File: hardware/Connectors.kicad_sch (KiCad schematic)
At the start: 9 parts, among them J1 USB_C_Receptacle_USB2.0, J14 Conn_01x05, J16 Harw_Conn_2x13, J2 Harw_Conn_1x2, J3 Harw_Conn_1x2, J8 Harw_Conn_1x4

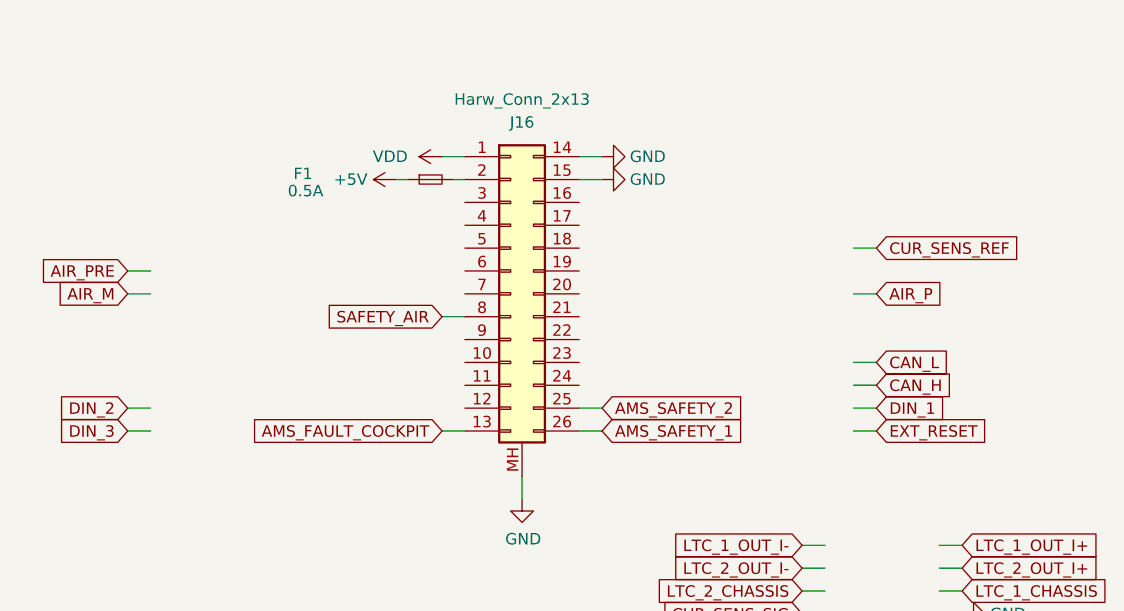
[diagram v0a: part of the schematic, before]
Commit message: pcb update
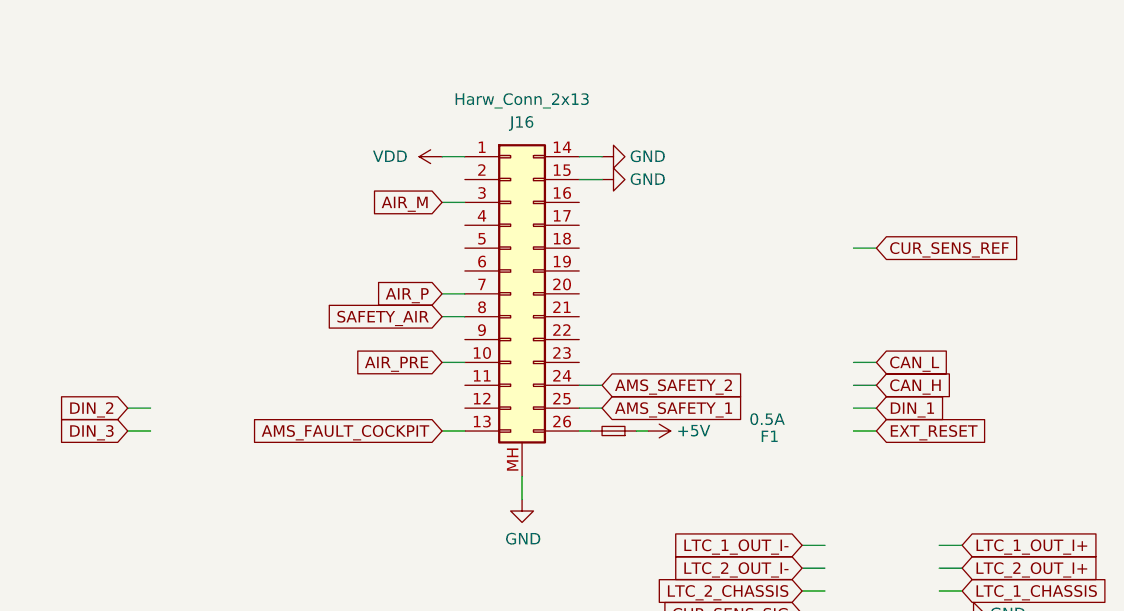
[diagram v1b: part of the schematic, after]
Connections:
- net AIR_M: now also J16.3
- net AIR_P: now also J16.7
- net AIR_PRE: now also J16.10
- net AMS_SAFETY_1: now also J16.25; no longer J16.26
- net AMS_SAFETY_2: now also J16.24; no longer J16.25
- net at F1.2: now also J16.26; no longer J16.2
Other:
- moved on the sheet: F1
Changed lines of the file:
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@@
     (stroke (width 0) (type default) (color 0 0 0 0))
   )
-  (wire (pts (xy 84.455 127) (xy 81.915 127))
+  (wire (pts (xy 84.455 124.46) (xy 81.915 124.46))
     (stroke (width 0) (type default) (color 0 0 0 0))
   )
@@
     (stroke (width 1) (type default) (color 132 0 0 1))
   )
-  (wire (pts (xy 62.865 99.06) (xy 61.595 99.06))
+  (wire (pts (xy 88.265 127) (xy 89.535 127))
     (stroke (width 0) (type default) (color 0 0 0 0))
   )
@@
     (stroke (width 0) (type default) (color 0 0 0 0))
   )
-  (wire (pts (xy 34.29 111.76) (xy 31.75 111.76))
+  (wire (pts (xy 69.215 101.6) (xy 66.675 101.6))
     (stroke (width 0) (type default) (color 0 0 0 0))
   )
@@
     (stroke (width 0) (type default) (color 0 0 0 0))
   )
-  (wire (pts (xy 34.29 109.22) (xy 31.75 109.22))
+  (wire (pts (xy 69.215 119.38) (xy 66.675 119.38))
     (stroke (width 0) (type default) (color 0 0 0 0))
   )
@@
     (stroke (width 0) (type default) (color 0 0 0 0))
   )
-  (wire (pts (xy 69.215 99.06) (xy 67.945 99.06))
+  (wire (pts (xy 81.915 127) (xy 83.185 127))
     (stroke (width 0) (type default) (color 0 0 0 0))
   )
@@
     (stroke (width 0) (type default) (color 0 0 0 0))
   )
-  (wire (pts (xy 112.395 111.76) (xy 114.935 111.76))
+  (wire (pts (xy 69.215 111.76) (xy 66.675 111.76))
     (stroke (width 0) (type default) (color 0 0 0 0))
   )
@@
     (stroke (width 0) (type default) (color 0 0 0 0))
   )
-  (wire (pts (xy 81.915 124.46) (xy 84.455 124.46))
+  (wire (pts (xy 81.915 121.92) (xy 84.455 121.92))
     (stroke (width 0) (type default) (color 0 0 0 0))
   )
@@
     )
   )
-  (global_label "AIR_PRE" (shape input) (at 31.75 109.22 180) (fields_autoplaced)
-    (effects (font (size 1.27 1.27)) (justify right))
-    (property "Intersheet References" "${INTERSHEET_REFS}" (id 0) (at 21.8058 109.2994 0)
+  (global_label "AIR_PRE" (shape input) (at 66.675 119.38 180) (fields_autoplaced)
+    (effects (font (size 1.27 1.27)) (justify right))
+    (property "Intersheet References" "${INTERSHEET_REFS}" (id 0) (at 56.7308 119.4594 0)
       (effects (font (size 1.27 1.27)) (justify right) hide)
     )
@@
     )
   )
-  (global_label "AMS_SAFETY_2" (shape input) (at 84.455 124.46 0) (fields_autoplaced)
+  (global_label "AMS_SAFETY_2" (shape input) (at 84.455 121.92 0) (fields_autoplaced)
+    (effects (font (size 1.27 1.27)) (justify left))
+    (property "Intersheet References" "${INTERSHEET_REFS}" (id 0) (at 100.2654 121.9994 0)
+      (effects (font (size 1.27 1.27)) (justify left) hide)
+    )
+  )
+  (global_label "SWDIO" (shape input) (at 178.435 142.24 180) (fields_autoplaced)
+    (effects (font (size 1.27 1.27)) (justify right))
+    (property "Intersheet References" "${INTERSHEET_REFS}" (id 0) (at 170.2446 142.1606 0)
+      (effects (font (size 1.27 1.27)) (justify right) hide)
+    )
+  )
+  (global_label "AIR_M" (shape input) (at 66.675 101.6 180) (fields_autoplaced)
+    (effects (font (size 1.27 1.27)) (justify right))
+    (property "Intersheet References" "${INTERSHEET_REFS}" (id 0) (at 58.9684 101.6794 0)
+      (effects (font (size 1.27 1.27)) (justify right) hide)
+    )
+  )
+  (global_label "AMS_SAFETY_1" (shape input) (at 84.455 124.46 0) (fields_autoplaced)
     (effects (font (size 1.27 1.27)) (justify left))
     (property "Intersheet References" "${INTERSHEET_REFS}" (id 0) (at 100.2654 124.5394 0)
@@
     )
   )
-  (global_label "SWDIO" (shape input) (at 178.435 142.24 180) (fields_autoplaced)
-    (effects (font (size 1.27 1.27)) (justify right))
-    (property "Intersheet References" "${INTERSHEET_REFS}" (id 0) (at 170.2446 142.1606 0)
-      (effects (font (size 1.27 1.27)) (justify right) hide)
-    )
-  )
-  (global_label "AIR_M" (shape input) (at 31.75 111.76 180) (fields_autoplaced)
-    (effects (font (size 1.27 1.27)) (justify right))
-    (property "Intersheet References" "${INTERSHEET_REFS}" (id 0) (at 24.0434 111.8394 0)
-      (effects (font (size 1.27 1.27)) (justify right) hide)
-    )
-  )
-  (global_label "AMS_SAFETY_1" (shape input) (at 84.455 127 0) (fields_autoplaced)
-    (effects (font (size 1.27 1.27)) (justify left))
-    (property "Intersheet References" "${INTERSHEET_REFS}" (id 0) (at 100.2654 127.0794 0)
-      (effects (font (size 1.27 1.27)) (justify left) hide)
-    )
-  )
   (global_label "D+" (shape input) (at 253.365 114.3 0) (fields_autoplaced)
     (effects (font (size 1.27 1.27)) (justify left))
@@
     )
   )
-  (global_label "AIR_P" (shape input) (at 114.935 111.76 0) (fields_autoplaced)
-    (effects (font (size 1.27 1.27)) (justify left))
-    (property "Intersheet References" "${INTERSHEET_REFS}" (id 0) (at 122.4602 111.6806 0)
-      (effects (font (size 1.27 1.27)) (justify left) hide)
+  (global_label "AIR_P" (shape input) (at 66.675 111.76 180) (fields_autoplaced)
+    (effects (font (size 1.27 1.27)) (justify right))
+    (property "Intersheet References" "${INTERSHEET_REFS}" (id 0) (at 59.1498 111.8394 0)
+      (effects (font (size 1.27 1.27)) (justify right) hide)
     )
   )
@@
     )
   )
-  (symbol (lib_id "Device:Fuse_Small") (at 65.405 99.06 0) (unit 1)
-    (in_bom yes) (on_board yes)
-    (property "Reference" "F1" (id 0) (at 50.165 98.425 0)
+  (symbol (lib_id "Device:Fuse_Small") (at 85.725 127 180) (unit 1)
+    (in_bom yes) (on_board yes)
+    (property "Reference" "F1" (id 0) (at 104.14 127.635 0)
       (effects (font (size 1.27 1.27)) (justify left))
     )
-    (property "Value" "0.5A" (id 1) (at 49.53 100.33 0)
+    (property "Value" "0.5A" (id 1) (at 104.775 125.73 0)
       (effects (font (size 1.27 1.27)) (justify left))
     )
-    (property "Footprint" "Fuse:Fuse_1206_3216Metric" (id 2) (at 65.405 99.06 0)
-      (effects (font (size 1.27 1.27)) hide)
-    )
-    (property "Datasheet" "~" (id 3) (at 65.405 99.06 0)
+    (property "Footprint" "Fuse:Fuse_1206_3216Metric" (id 2) (at 85.725 127 0)
+      (effects (font (size 1.27 1.27)) hide)
+    )
+    (property "Datasheet" "~" (id 3) (at 85.725 127 0)
       (effects (font (size 1.27 1.27)) hide)
     )
@@
     (pin "1")
   )
-  (symbol (lib_id "power:+5V") (at 61.595 99.06 90) (unit 1)
-    (in_bom yes) (on_board yes)
-    (property "Reference" "#PWR03" (id 0) (at 65.405 99.06 0)
-      (effects (font (size 1.27 1.27)) hide)
-    )
-    (property "Value" "+5V" (id 1) (at 56.515 99.06 90))
-    (property "Footprint" "" (id 2) (at 61.595 99.06 0)
-      (effects (font (size 1.27 1.27)) hide)
-    )
-    (property "Datasheet" "" (id 3) (at 61.595 99.06 0)
-      (effects (font (size 1.27 1.27)) hide)
-    )
+  (symbol (lib_id "power:+5V") (at 89.535 127 270) (unit 1)
+    (in_bom yes) (on_board yes)
+    (property "Reference" "#PWR03" (id 0) (at 85.725 127 0)
+      (effects (font (size 1.27 1.27)) hide)
+    )
+    (property "Value" "+5V" (id 1) (at 94.615 127 90))
+    (property "Footprint" "" (id 2) (at 89.535 127 0)
+      (effects (font (size 1.27 1.27)) hide)
+    )
+    (property "Datasheet" "" (id 3) (at 89.535 127 0)
+      (effects (font (size 1.27 1.27)) hide)
+    )

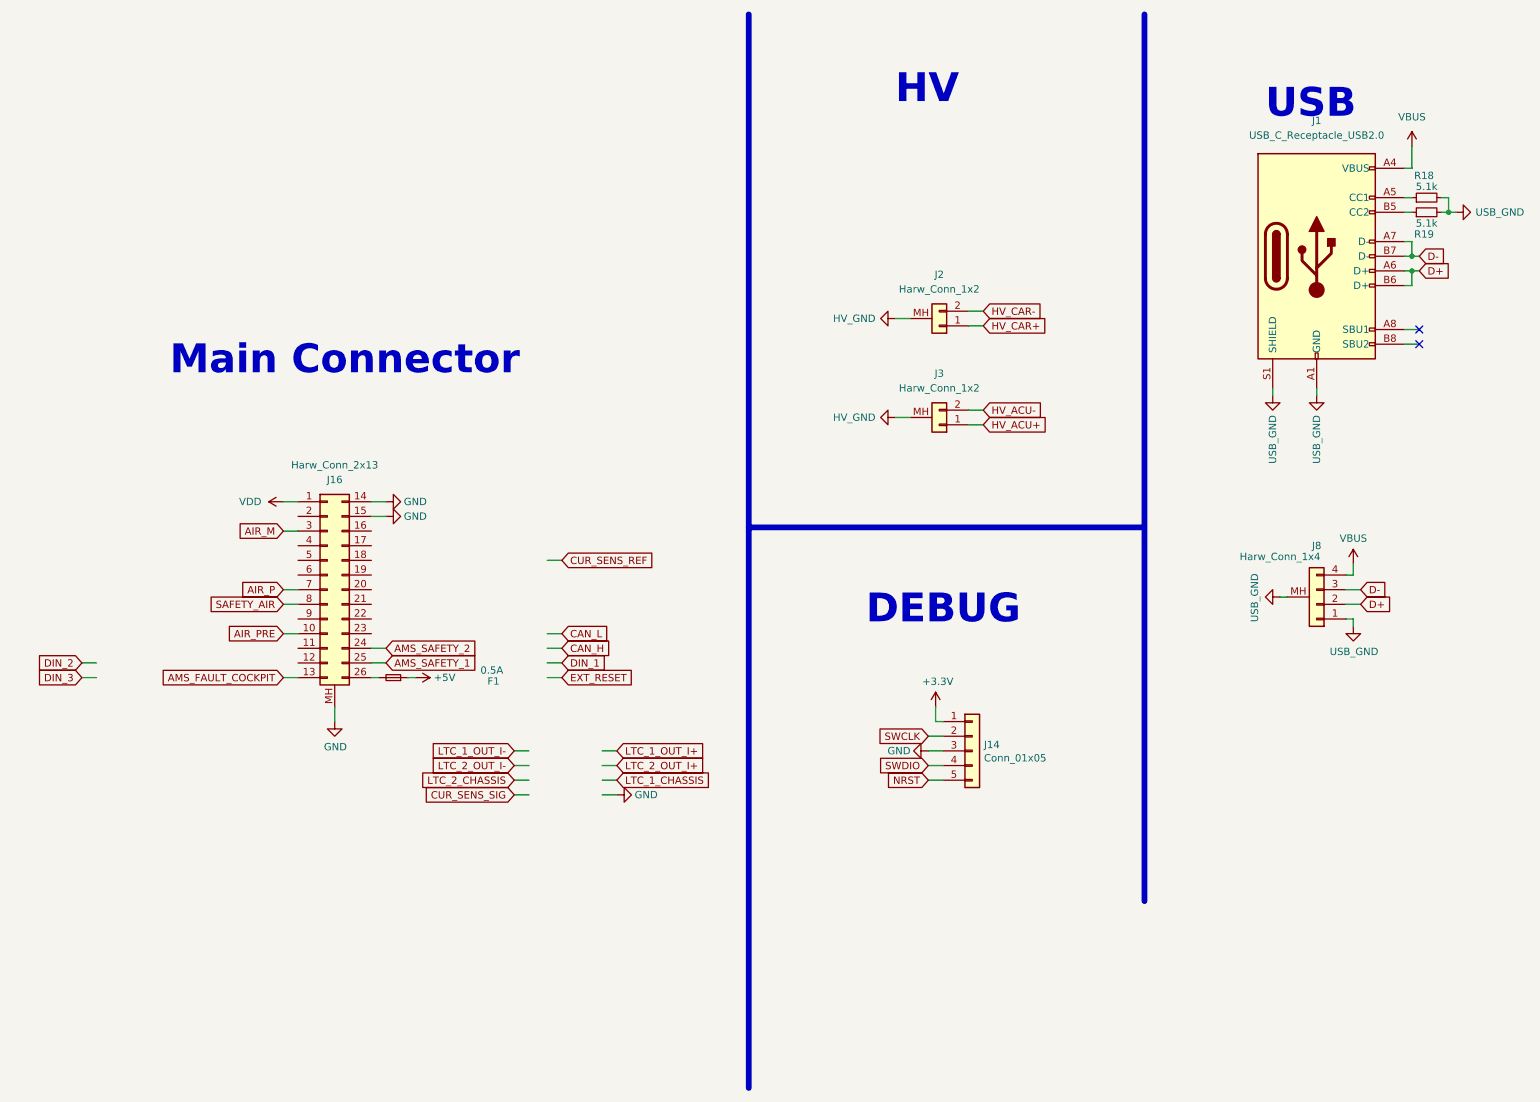
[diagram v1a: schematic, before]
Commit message: schemat sync
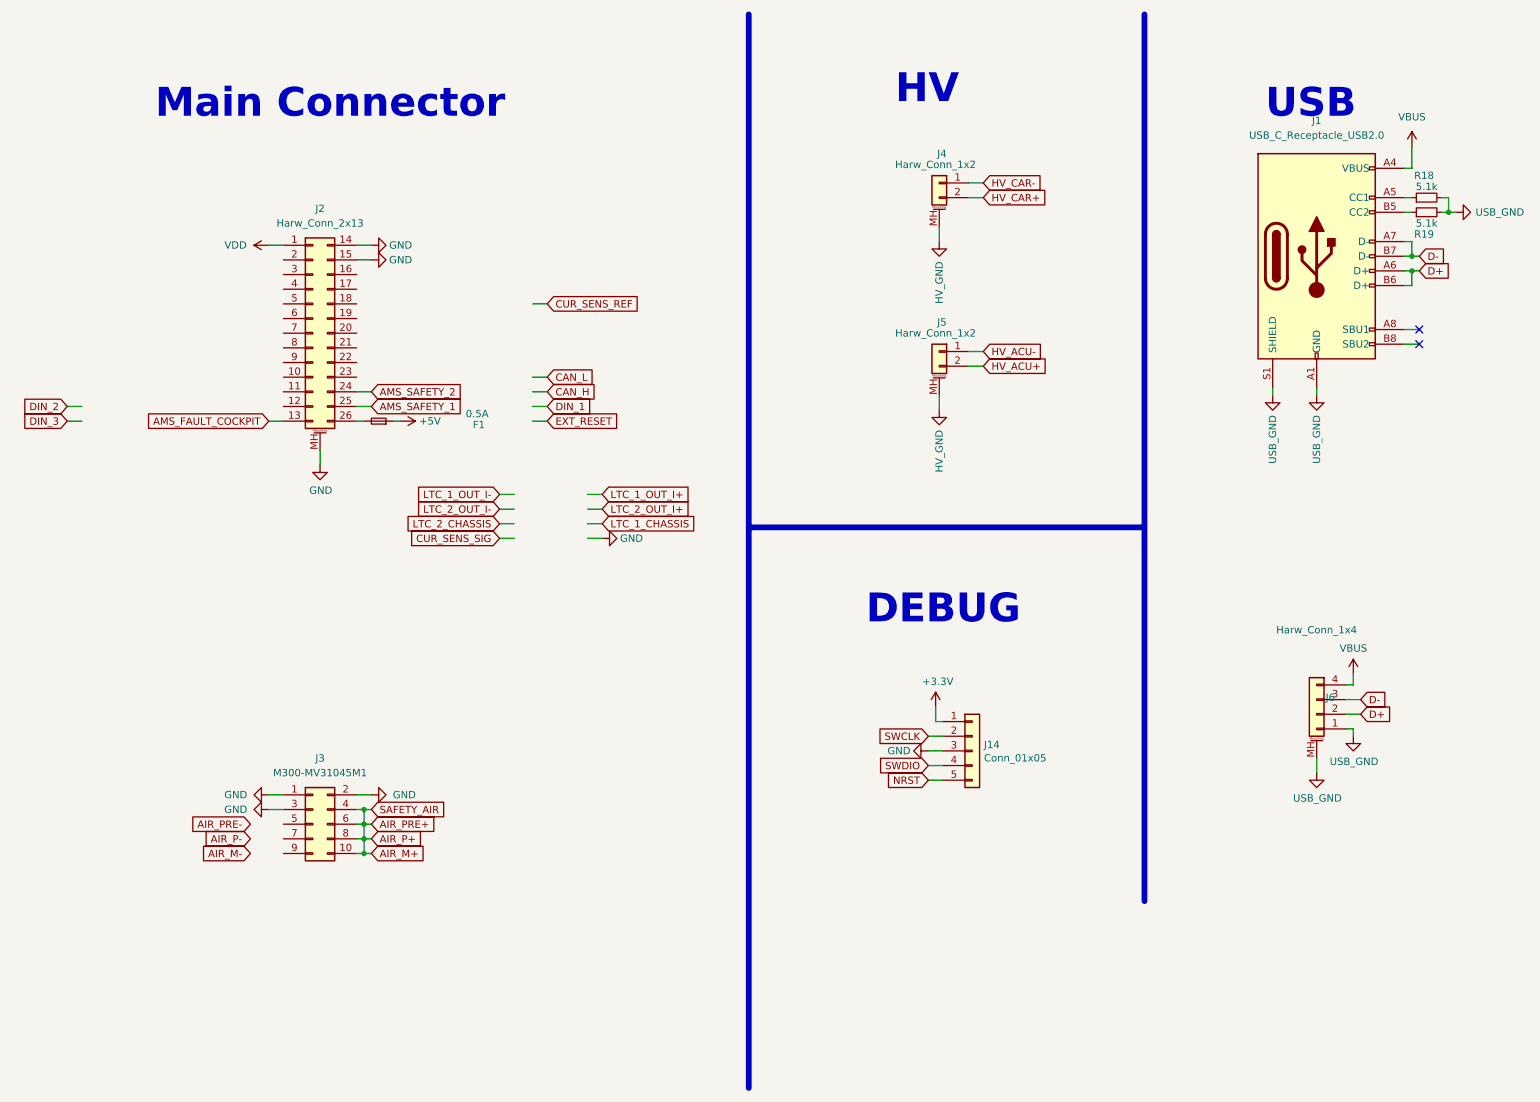
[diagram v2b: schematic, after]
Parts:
- removed J16: Harw_Conn_2x13, M80-85126YY, symbol Harwin 26 pin 90 deg:Harw_Conn_2x13
- removed J2: Harw_Conn_1x2, M808420245, symbol Harwin 2 pin 90 deg:Harw_Conn_1x2
- removed J3: Harw_Conn_1x2, Harwin 2 pin 90 deg:M808420245, symbol Harwin 2 pin 90 deg:Harw_Conn_1x2
- removed J8: Harw_Conn_1x4, M80-8420445, symbol Harwin 4 pin 90 deg:Harw_Conn_1x4
- added J2: Harw_Conn_2x13, M80-85126YY, symbol Harwin 26 pin 90 deg:Harw_Conn_2x13
- added J3: M300-MV31045M1, M300MV31045M1, symbol M300-MV31045M1:M300-MV31045M1
- added J4, J5: Harw_Conn_1x2, M808420245, symbol Harwin 2 pin 90 deg:Harw_Conn_1x2
- added J6: Harw_Conn_1x4, M80-8420445, symbol Harwin 4 pin 90 deg:Harw_Conn_1x4
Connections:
- net AMS_FAULT_COCKPIT: now also J2.13
- net AMS_SAFETY_1: now also J2.25
- net AMS_SAFETY_2: now also J2.24
- net D+: now also J6.2
- net D-: now also J6.3
- net GND: now also J2.14, J2.15, J2.MH, J3.1, J3.2, J3.3
- net HV_ACU+: now also J5.2
- net HV_ACU-: now also J5.1
- net HV_CAR+: now also J4.2
- net HV_CAR-: now also J4.1
- net ISO_GND: now also J4.MH, J5.MH
- net USB_GND: now also J6.1, J6.MH
- net VBUS: now also J6.4
- net VDD: now also J2.1
- net at F1.2: now also J2.26
- new net AIR_M+: J3.10, J3.4, J3.6, J3.8
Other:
- moved on the sheet: F1
